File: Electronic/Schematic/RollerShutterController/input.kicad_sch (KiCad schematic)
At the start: 17 parts, among them U4 LTV-247

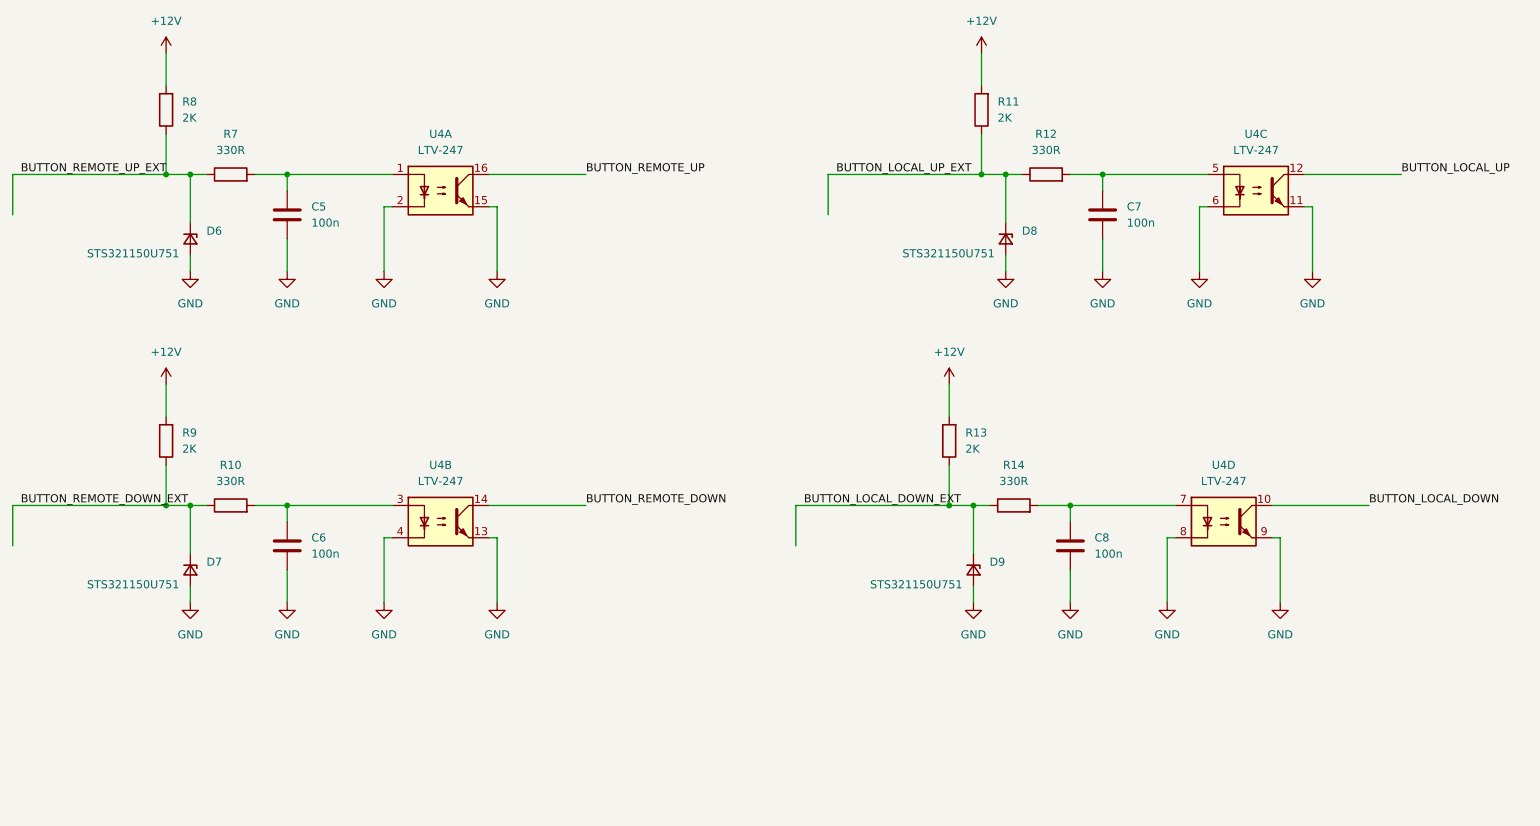
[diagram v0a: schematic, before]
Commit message: Added electronic project.
Signed-off-by: Kamil Lazowski <autobrewing@gmail.com>
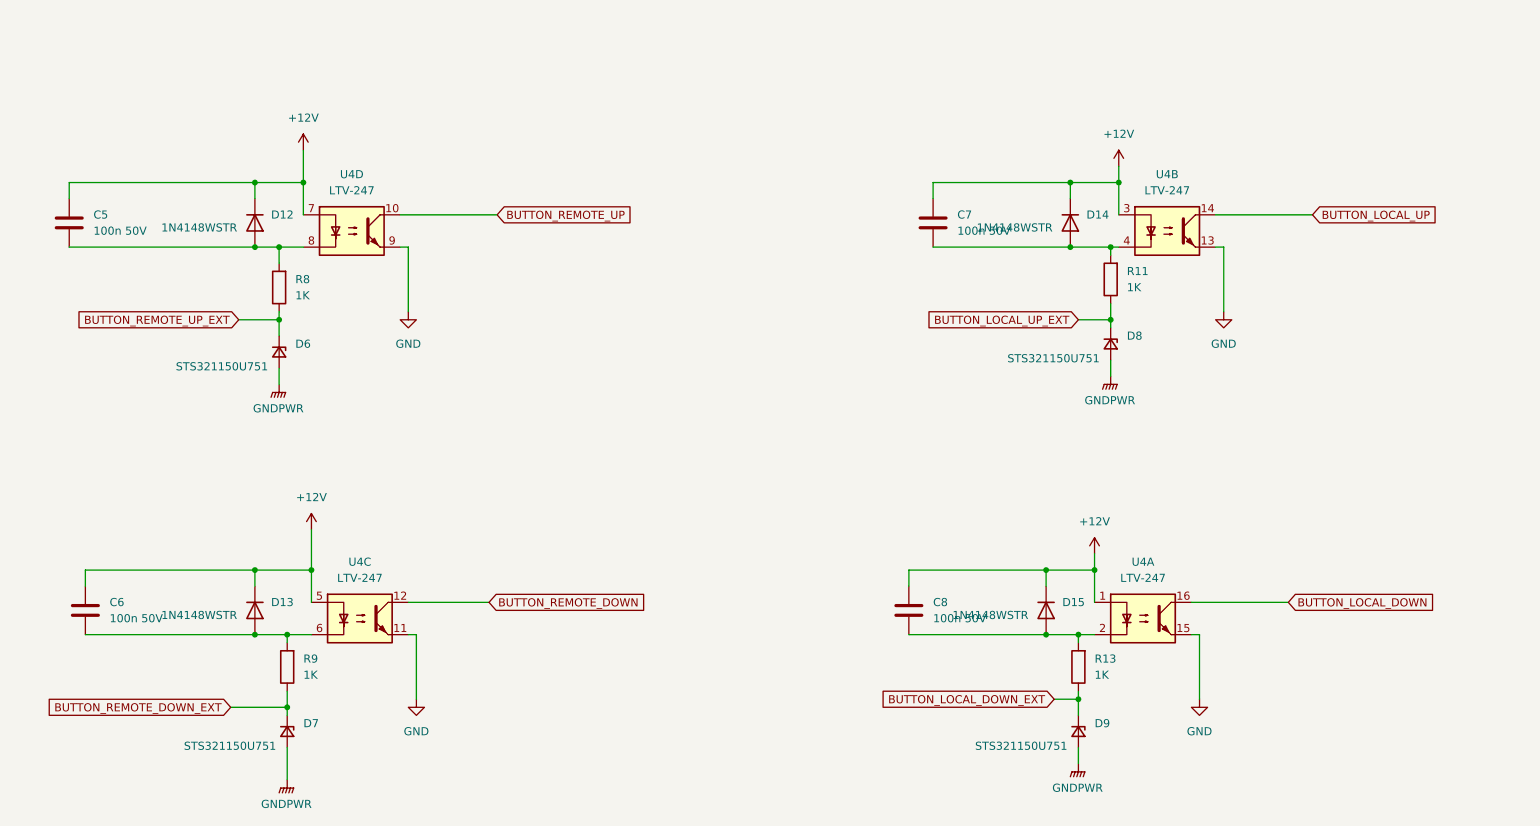
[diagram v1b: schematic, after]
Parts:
- removed R10, R12, R14, R7: 330R, symbol Device:R
- added D12, D13, D14, D15: 1N4148WSTR, Diode_SMD:D_SOD-323_HandSoldering, symbol Diode:1N4148WS
- C5, C6, C7, C8: value 100n -> 100n 50V; footprint (none) -> Capacitor_SMD:C_0603_1608Metric_Pad1.08x0.95mm_HandSolder
- D6, D7, D8, D9: footprint Diode_SMD:D_SOD-323F -> Diode_SMD:D_SOD-323_HandSoldering
- R11, R13, R8, R9: value 2K -> 1K; footprint (none) -> Resistor_SMD:R_1206_3216Metric_Pad1.30x1.75mm_HandSolder
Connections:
- net +12V: now also C5.1, C6.1, C7.1, C8.1, U4.1, U4.3, U4.5, U4.7, D12.1 (K), D13.1 (K), D14.1 (K), D15.1 (K); no longer R11.2, R13.2, R8.2, R9.2
- net BUTTON_LOCAL_DOWN: now also U4.16; no longer U4.10
- net BUTTON_LOCAL_UP: now also U4.14; no longer U4.12
- net BUTTON_REMOTE_DOWN: now also U4.12; no longer U4.14
- net BUTTON_REMOTE_UP: now also U4.10; no longer U4.16
- net GND: no longer C5.2, C6.2, C7.2, C8.2, D6.2 (A), D7.2 (A), D8.2 (A), D9.2 (A), U4.2, U4.4, U4.6, U4.8
- new net: C7.2, D14.2 (A), R11.2, U4.4
- new net: C5.2, D12.2 (A), R8.2, U4.8
- new net: C8.2, D15.2 (A), R13.2, U4.2
- new net: C6.2, D13.2 (A), R9.2, U4.6
- new net GNDPWR: D6.2 (A), D7.2 (A), D8.2 (A), D9.2 (A)
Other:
- moved on the sheet: C5, C6, C7, C8, D6, D7, D8, D9, R11, R13, R8, R9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
